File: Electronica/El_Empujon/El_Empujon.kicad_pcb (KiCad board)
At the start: 2 copper layers, 86 x 85 mm, 28 parts, among them J1 Screw_Terminal_01x02, J10 Conn_01x03_Socket, J11 Conn_01x05_Socket, J12 Conn_01x05_Socket, J13 Conn_01x05_Socket, J2 Conn_01x04_Socket, J3 Conn_01x19_Socket, J4 Conn_01x19_Socket, J5 Conn_01x08_Socket, J6 Conn_01x04_Socket, J7 Conn_01x08_Socket, J8 Conn_01x04_Socket, J9 Conn_01x03_Socket, U1 AMS1117-3.3

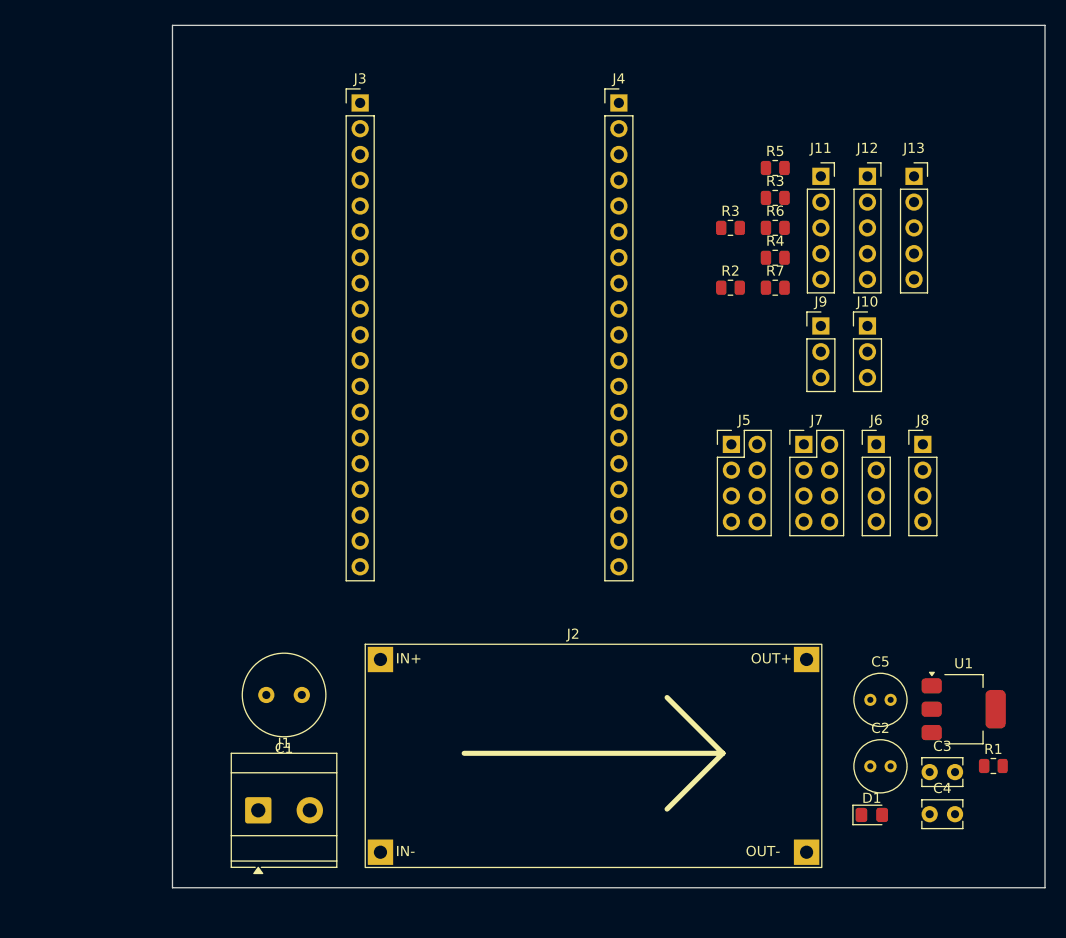
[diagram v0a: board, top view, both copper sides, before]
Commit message: Generacion del STEP, finalizacion del esquematico y de la PCB, generacion de los archivos de manufactura de la PCB, Pedido de la PCB y actualizacion del Presupuesto.
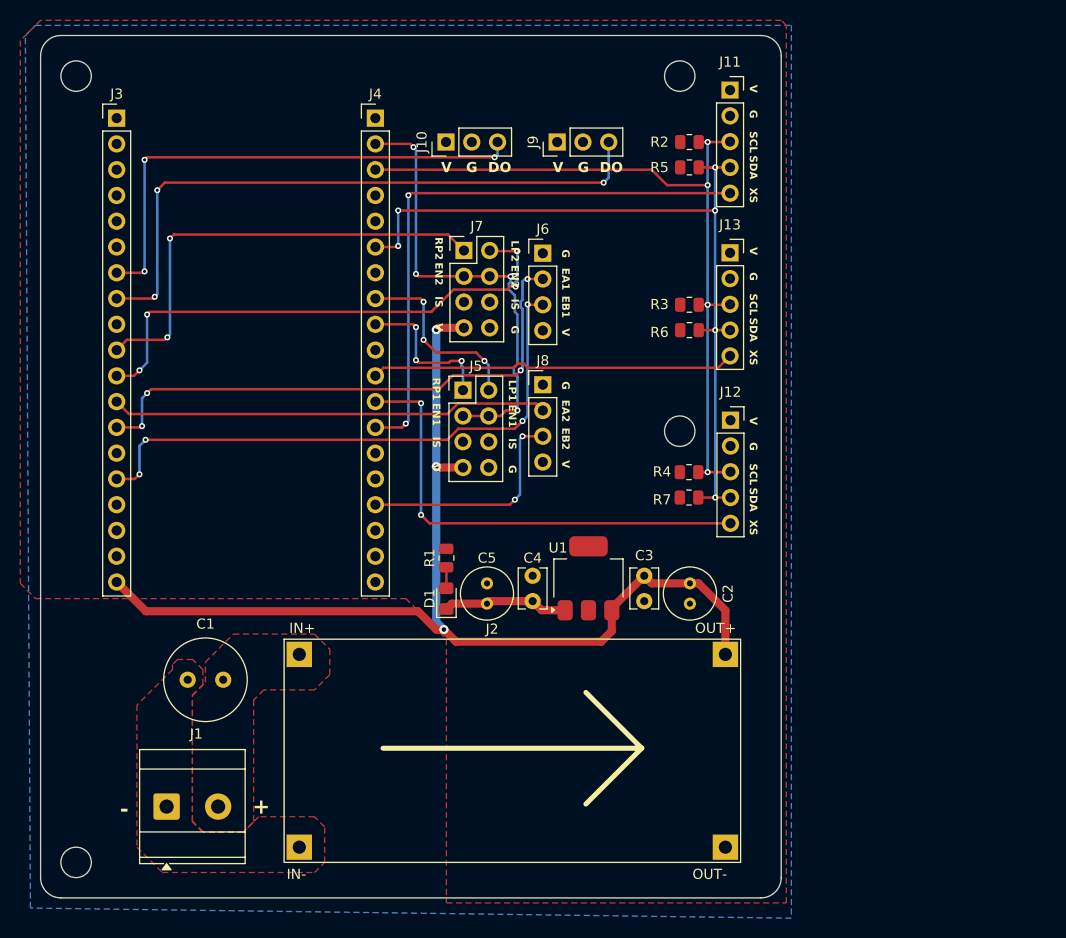
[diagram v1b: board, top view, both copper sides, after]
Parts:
- removed the R3 at (142.0, 65.0)
- moved R1 57.7 mm to (114.0, 97.5), turned to 90 degrees
- moved D1 47.0 mm to (114.0, 101.5), turned to 90 degrees
- moved C4 45.6 mm to (122.5, 99.2), turned to -90 degrees
- moved J10 45.3 mm to (114.0, 56.5), turned to 90 degrees
- moved C5 39.5 mm to (118.0, 100.0), turned to -90 degrees
- moved U1 39.2 mm to (128.0, 99.5), turned to 90 degrees
- moved J7 38.6 mm to (115.7, 67.2)
- moved J8 37.9 mm to (123.5, 80.4)
- moved J6 37.9 mm to (123.5, 67.5)
- moved C3 34.1 mm to (133.5, 99.2), turned to -90 degrees
- moved J9 31.7 mm to (124.9, 56.5), turned to 90 degrees
- moved J12 27.6 mm to (142.0, 83.9)
- moved J5 27.0 mm to (115.6, 81.0)
- moved C2 25.3 mm to (138.0, 100.0), turned to -90 degrees
- moved J3 24.0 mm to (81.5, 54.1)
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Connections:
- net Net-(J1-Pin_1) renamed GND2
- net Net-(J1-Pin_2) renamed +11V1
- C2 pad 1: /Alimentacion/5V -> +5V
- C2 pad 2: /Alimentacion/GND -> GND
- C3 pad 1: /Alimentacion/5V -> +5V
- C3 pad 2: /Alimentacion/GND -> GND
- C4 pad 1: /Alimentacion/3.3V -> +3V3
- C4 pad 2: /Alimentacion/GND -> GND
- C5 pad 1: /Alimentacion/3.3V -> +3V3
- C5 pad 2: /Alimentacion/GND -> GND
- D1 pad 1: /Alimentacion/GND -> GND
- J10 pad 1: /VL53L0X y TCRT5000/IFV -> +3V3
- J10 pad 2: /VL53L0X y TCRT5000/GND -> GND
- J10 pad 3: /VL53L0X y TCRT5000/IFDO2 -> /Esp32/GPIO32
- J11 pad 1: /VL53L0X y TCRT5000/TOFV -> +3V3
- J11 pad 2: /VL53L0X y TCRT5000/GND -> GND
- J11 pad 3: /VL53L0X y TCRT5000/TOFSCL -> /Esp32/GPIO22
- J11 pad 4: /VL53L0X y TCRT5000/TOFSDA -> /Esp32/GPIO21
- J11 pad 5: /VL53L0X y TCRT5000/TOFXSHUT1 -> /Esp32/GPIO4
- J12 pad 1: /VL53L0X y TCRT5000/TOFV -> +3V3
- J12 pad 2: /VL53L0X y TCRT5000/GND -> GND
- J12 pad 3: /VL53L0X y TCRT5000/TOFSCL -> /Esp32/GPIO22
- J12 pad 4: /VL53L0X y TCRT5000/TOFSDA -> /Esp32/GPIO21
- J12 pad 5: /VL53L0X y TCRT5000/TOFXSHUT2 -> /Esp32/GPIO16
- J13 pad 1: /VL53L0X y TCRT5000/TOFV -> +3V3
- J13 pad 2: /VL53L0X y TCRT5000/GND -> GND
- J13 pad 3: /VL53L0X y TCRT5000/TOFSCL -> /Esp32/GPIO22
- J13 pad 4: /VL53L0X y TCRT5000/TOFSDA -> /Esp32/GPIO21
- J13 pad 5: /VL53L0X y TCRT5000/TOFXSHUT3 -> /Esp32/GPIO17
- J2 pad 3: /Alimentacion/5V -> +5V
- J2 pad 4: /Alimentacion/GND -> GND
- J3 pad 10: /Esp32/GPIO26 -> /BTS7960/RPWM2
- J3 pad 11: /Esp32/GPIO27 -> /BTS7960/LPWM2
- J3 pad 12: /Esp32/GPIO14 -> /BTS7960/ENCA2
- J3 pad 13: /Esp32/GPIO12 -> /BTS7960/ENCA1
- J3 pad 14: /Esp32/GND -> GND
- J3 pad 15: /Esp32/GPIO13 -> /BTS7960/ENCB1
- J3 pad 19: /Esp32/5V -> +5V
- J4 pad 1: /Esp32/GND -> GND
- J4 pad 16: /Esp32/GPIO15 -> /BTS7960/ENCB2
- J4 pad 2: /Esp32/GPIO23 -> /BTS7960/L_EN1
- J4 pad 7: /Esp32/GND -> GND
- J4 pad 8: /Esp32/GPIO19 -> /BTS7960/LPWM1
- J4 pad 9: /Esp32/GPIO18 -> /BTS7960/RPWM1
- J5 pad 3: /BTS7960/R_EN1 -> /BTS7960/L_EN1
- J5 pad 7: /BTS7960/VCC -> +5V
- J5 pad 8: /BTS7960/GND -> GND
- J6 pad 1: /BTS7960/GND -> GND
- J6 pad 4: /BTS7960/VCC -> +3V3
- J7 pad 3: /BTS7960/R_EN2 -> /BTS7960/L_EN1
- J7 pad 4: /BTS7960/L_EN2 -> /BTS7960/L_EN1
- J7 pad 7: /BTS7960/VCC -> +5V
- J7 pad 8: /BTS7960/GND -> GND
- J8 pad 1: /BTS7960/GND -> GND
- J8 pad 4: /BTS7960/VCC -> +3V3
- J9 pad 1: /VL53L0X y TCRT5000/IFV -> +3V3
- J9 pad 2: /VL53L0X y TCRT5000/GND -> GND
- J9 pad 3: /VL53L0X y TCRT5000/IFDO1 -> /Esp32/GPIO33
- R1 pad 2: /Alimentacion/3.3V -> +3V3
- R2 pad 1: /VL53L0X y TCRT5000/TOFV -> +3V3
- R2 pad 2: /VL53L0X y TCRT5000/TOFSCL -> /Esp32/GPIO22
- R3 pad 1: /VL53L0X y TCRT5000/TOFV -> +3V3
- R3 pad 2: /VL53L0X y TCRT5000/TOFSCL -> /Esp32/GPIO22
- R4 pad 1: /VL53L0X y TCRT5000/TOFV -> +3V3
- R4 pad 2: /VL53L0X y TCRT5000/TOFSCL -> /Esp32/GPIO22
- R5 pad 1: /VL53L0X y TCRT5000/TOFV -> +3V3
- R5 pad 2: /VL53L0X y TCRT5000/TOFSDA -> /Esp32/GPIO21
- R6 pad 1: /VL53L0X y TCRT5000/TOFV -> +3V3
- R6 pad 2: /VL53L0X y TCRT5000/TOFSDA -> /Esp32/GPIO21
- R7 pad 1: /VL53L0X y TCRT5000/TOFV -> +3V3
- R7 pad 2: /VL53L0X y TCRT5000/TOFSDA -> /Esp32/GPIO21
- U1 pad 1: /Alimentacion/GND -> GND
- U1 pad 2: /Alimentacion/3.3V -> +3V3
- U1 pad 3: /Alimentacion/5V -> +5V
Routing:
- net +5V: track 0.00 -> 107.5 mm, vias 0 -> 3
- net /Esp32/GPIO21: track 0.00 -> 79.2 mm, vias 0 -> 6
- net /Esp32/GPIO22: track 0.00 -> 75.3 mm, vias 0 -> 4
- net /Esp32/GPIO33: track 0.00 -> 62.9 mm, vias 0 -> 3
- net /Esp32/GPIO4: track 0.00 -> 57.6 mm, vias 0 -> 2
- net /BTS7960/ENCB1: track 0.00 -> 57.2 mm, vias 0 -> 4
- net /BTS7960/ENCA1: track 0.00 -> 54.8 mm, vias 0 -> 4
- net /BTS7960/LPWM2: track 0.00 -> 52.1 mm, vias 0 -> 4
- net /Esp32/GPIO32: track 0.00 -> 50.0 mm, vias 0 -> 3
- net /Esp32/GPIO16: track 0.00 -> 46.4 mm, vias 0 -> 2
- net /BTS7960/L_EN1: track 0.00 -> 45.4 mm, vias 0 -> 4
- net /BTS7960/RPWM2: track 0.00 -> 45.2 mm, vias 0 -> 2
- net /BTS7960/ENCA2: track 0.00 -> 43.2 mm
- net /Esp32/GPIO17: track 0.00 -> 36.2 mm
- net /BTS7960/ENCB2: track 0.00 -> 22.5 mm, vias 0 -> 2
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- added copper zone on F.Cu, net +11V1
- added copper zone on F.Cu, net +3V3
- added copper zone on B.Cu, net GND
- added copper zone on F.Cu, net GND2
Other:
- board size 86 x 85 mm -> 73 x 85 mm
- board text added: "+"
- board text added: "-"
- board text added: "DO"
- board text added: "EA1"
- board text added: "EA2"
- board text added: "EB1"
- board text added: "EB2"
- board text added: "EL_Empujom_Hub 27/10/2026 v1.0"
- board text added: "EN1"
- board text added: "EN2"
- board text added: "G"
- board text added: "IS"
- board text added: "LP1"
- board text added: "LP2"
- board text added: "RP1"
- board text added: "RP2"
- board text added: "SCL"
- board text added: "SDA"
- board text added: "V"
- board text added: "XS"
- board text added: "make_by_BETA"
